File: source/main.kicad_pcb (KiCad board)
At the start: 2 copper layers, 85.6 x 54 mm, 61 parts, among them P1 USB_Type_C_Receptacle_16_pin

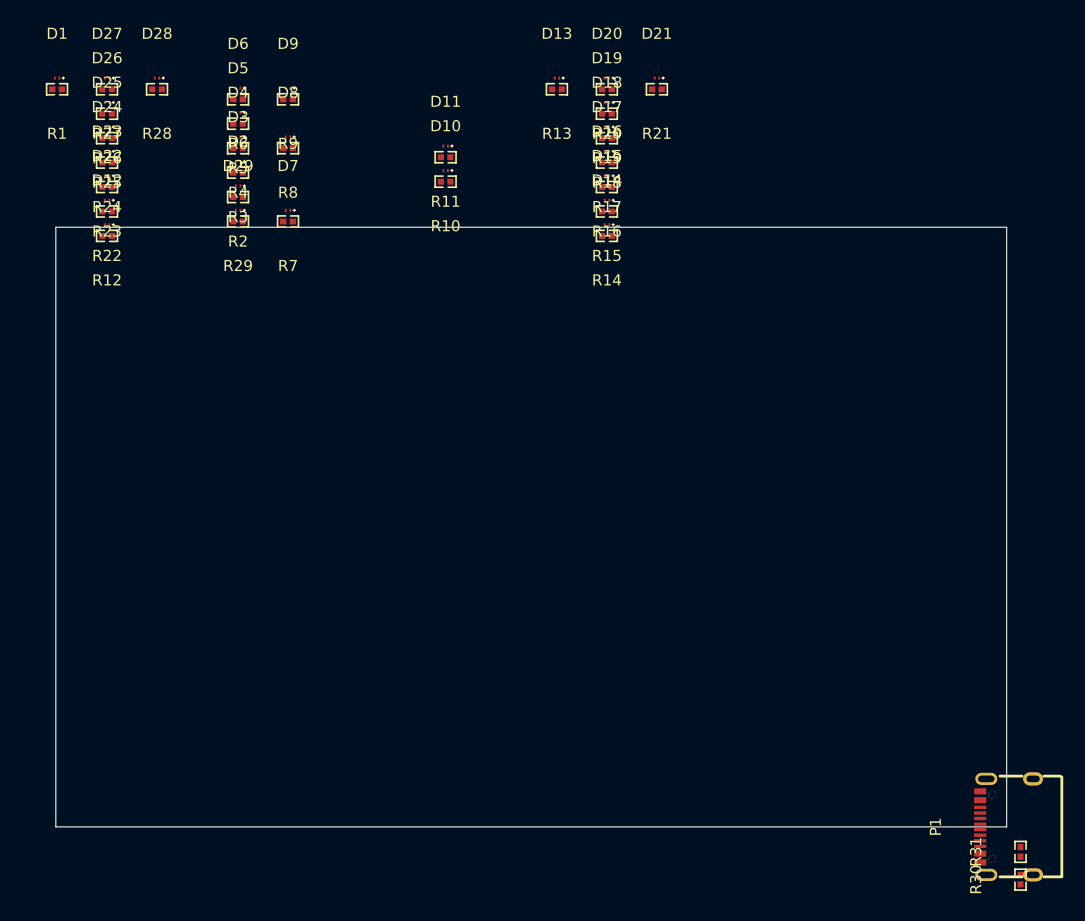
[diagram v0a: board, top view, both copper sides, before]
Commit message: wip:
- add outline with rounded corners
- add logo
- add more layout
- insert vias for vbus anode led
- move designators
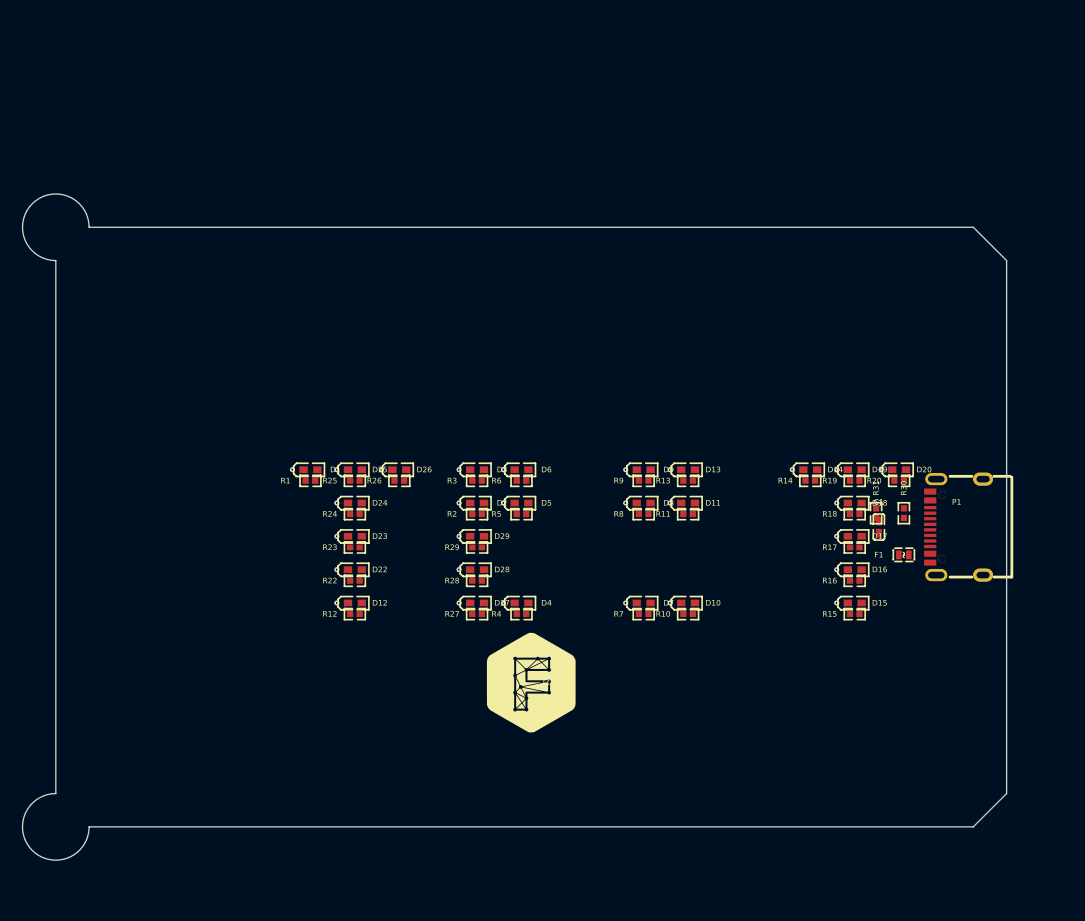
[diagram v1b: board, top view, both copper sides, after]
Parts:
- removed D21: LED, lcsc:LED-SMD_L0.65-W0.35-P0.41_XL-0201SURC
- removed R21: 100Ω, lcsc:R0402
- added C1: 100nF 16V X7R, lcsc:C0402, F.Cu at (74.1, 27.0)
- added F1: Fuse, lcsc:F0402, F.Cu at (76.3, 29.5)
- added LOGO1: Faebryk_Logo, logo:faebryk_logo, F.Cu at (42.8, 41.0)
- D1, D10, D11, D12, D13, D14, D15, D16, D17, D18, D19, D2, D20, D22, D23, D24, D25, D26, D27, D28, D29, D3, D4, D5, D6, D7, D8, D9: footprint lcsc:LED-SMD_L0.65-W0.35-P0.41_XL-0201SURC -> lcsc:LED0402-R-RD_RED
- moved D27 57.8 mm to (37.9, 33.8)
- moved R27 57.8 mm to (37.9, 34.8)
- moved D28 52.8 mm to (37.9, 30.8)
- moved R28 52.8 mm to (37.9, 31.8)
- moved D4 49.1 mm to (41.9, 33.8)
- moved R4 49.1 mm to (41.9, 34.8)
- moved D7 47.7 mm to (52.9, 33.8)
- moved R7 47.7 mm to (52.9, 34.8)
- moved D9 47.0 mm to (52.9, 21.8)
- moved R9 47.0 mm to (52.9, 22.8)
- moved D8 45.9 mm to (52.9, 24.8)
- moved R8 45.9 mm to (52.9, 25.8)
- moved D10 44.6 mm to (56.9, 33.8)
- moved R10 44.6 mm to (56.9, 34.8)
- moved D20 44.0 mm to (75.9, 21.8)
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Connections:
- net P1-11-P1-2 renamed F1-1-P1-11-P1-2
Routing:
- net D9-2: vias 0 -> 1
- net D8-2: vias 0 -> 1
- net D7-2: vias 0 -> 1
- net D6-2: vias 0 -> 1
- net D5-2: vias 0 -> 1
- net D4-2: vias 0 -> 1
- net D3-2: vias 0 -> 1
- net D29-2: vias 0 -> 1
- net D28-2: vias 0 -> 1
- net D27-2: vias 0 -> 1
- net D26-2: vias 0 -> 1
- net D25-2: vias 0 -> 1
- net D24-2: vias 0 -> 1
- net D23-2: vias 0 -> 1
- net D22-2: vias 0 -> 1
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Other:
- board size 85.6 x 54 mm -> 88.6 x 60 mm
